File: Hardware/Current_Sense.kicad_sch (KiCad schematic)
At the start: 39 parts, among them IC2 INA241A4IDR, IC3 AMC1350DWVR, J6 Scrut Conn, SW4 Scrut Select, U10 TLV9002QDRQ1, U9 REF35125QDBVR

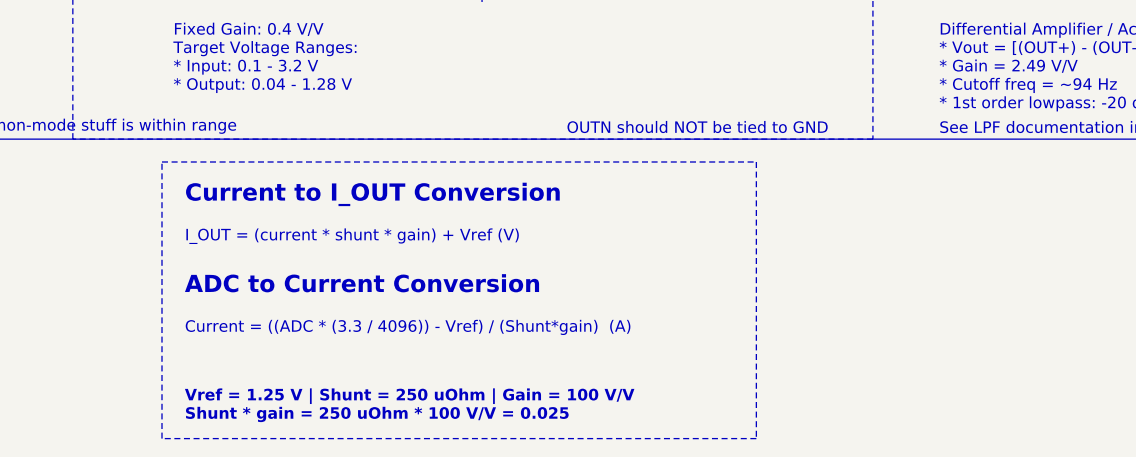
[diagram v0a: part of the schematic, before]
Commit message: starting routing i think
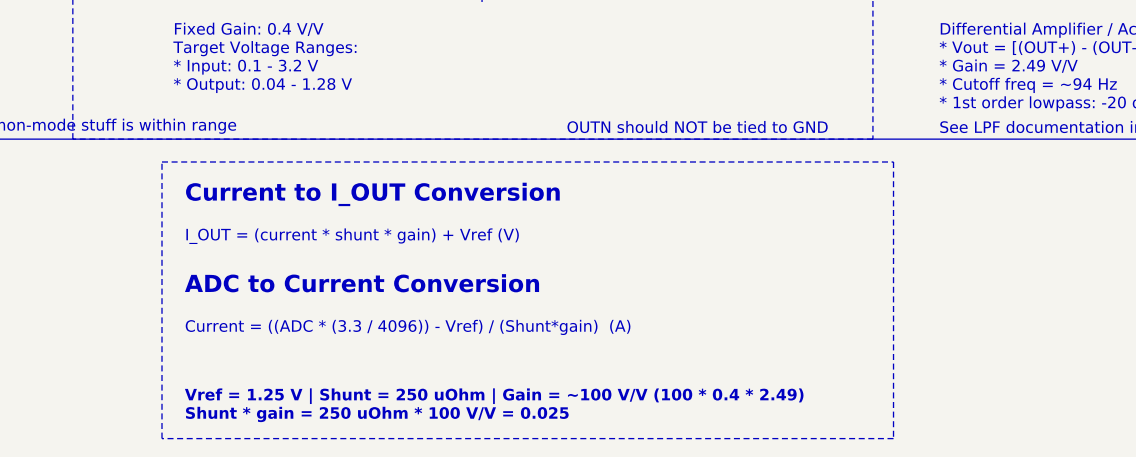
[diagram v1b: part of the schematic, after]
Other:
- note added: "Vref = 1.25 V | Shunt = 250 uOhm | Gain = ~100 V/V (100 * 0.4 * 2.49) Shunt * gain = 250 uOhm * 100 V/V = 0.025"
- note removed: "Vref = 1.25 V | Shunt = 250 uOhm | Gain = 100 V/V Shunt * gain = 250 uOhm * 100 V/V = 0.025"
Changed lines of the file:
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@@
 	(rectangle
 		(start 93.98 165.1)
-		(end 160.02 195.834)
+		(end 175.26 195.834)
 		(stroke
 			(width 0)
@@
 		)
 	)
-	(text "Vref = 1.25 V | Shunt = 250 uOhm | Gain = 100 V/V\nShunt * gain = 250 uOhm * 100 V/V = 0.025"
+	(text "Vref = 1.25 V | Shunt = 250 uOhm | Gain = ~100 V/V (100 * 0.4 * 2.49)\nShunt * gain = 250 uOhm * 100 V/V = 0.025"
 		(exclude_from_sim no)
 		(at 96.52 190.5 0)
